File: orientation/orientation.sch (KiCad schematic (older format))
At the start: 8 parts, among them J1 Conn_01x02, J2 Conn_01x04, SW1 SW_SPST, U1 Teensy4.0, U2 STSPIN220, U3 bno055

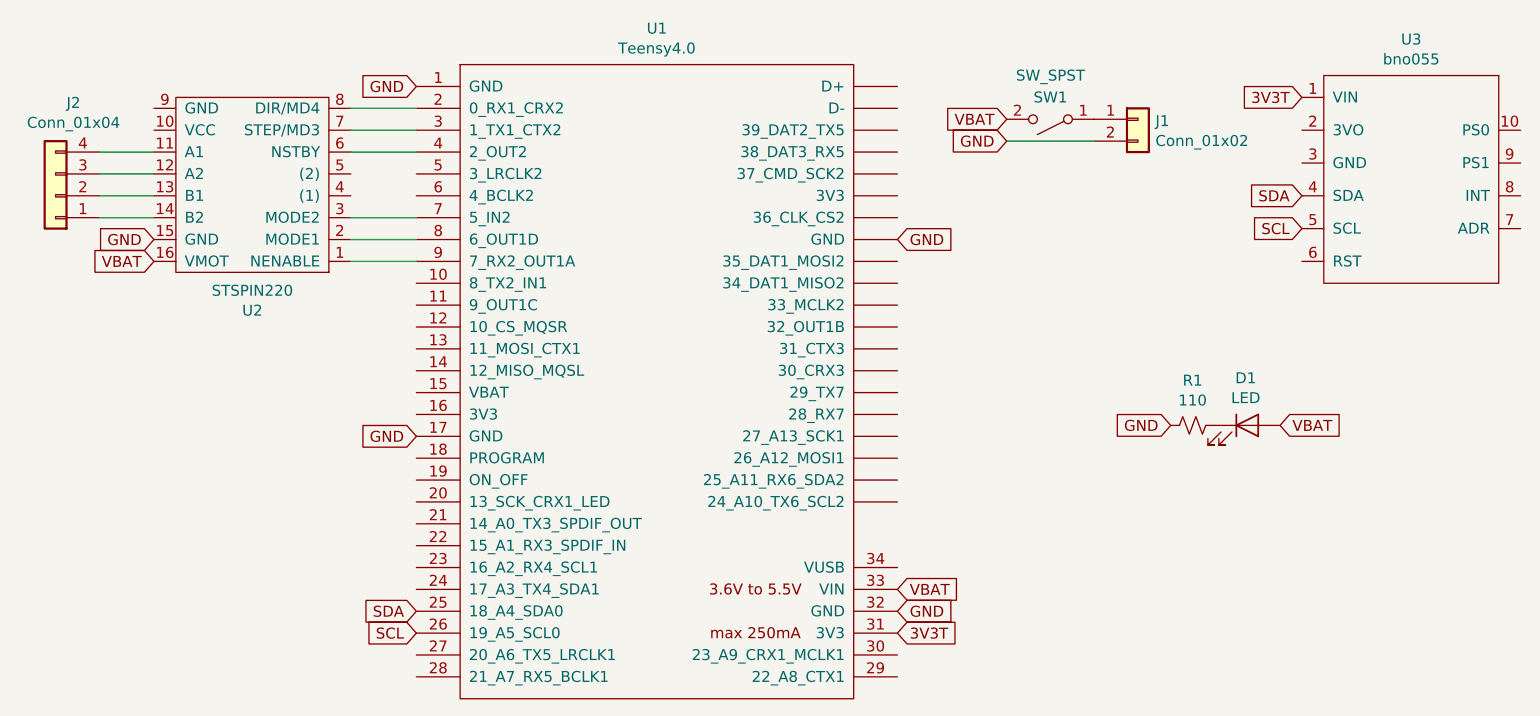
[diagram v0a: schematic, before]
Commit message: misc changes
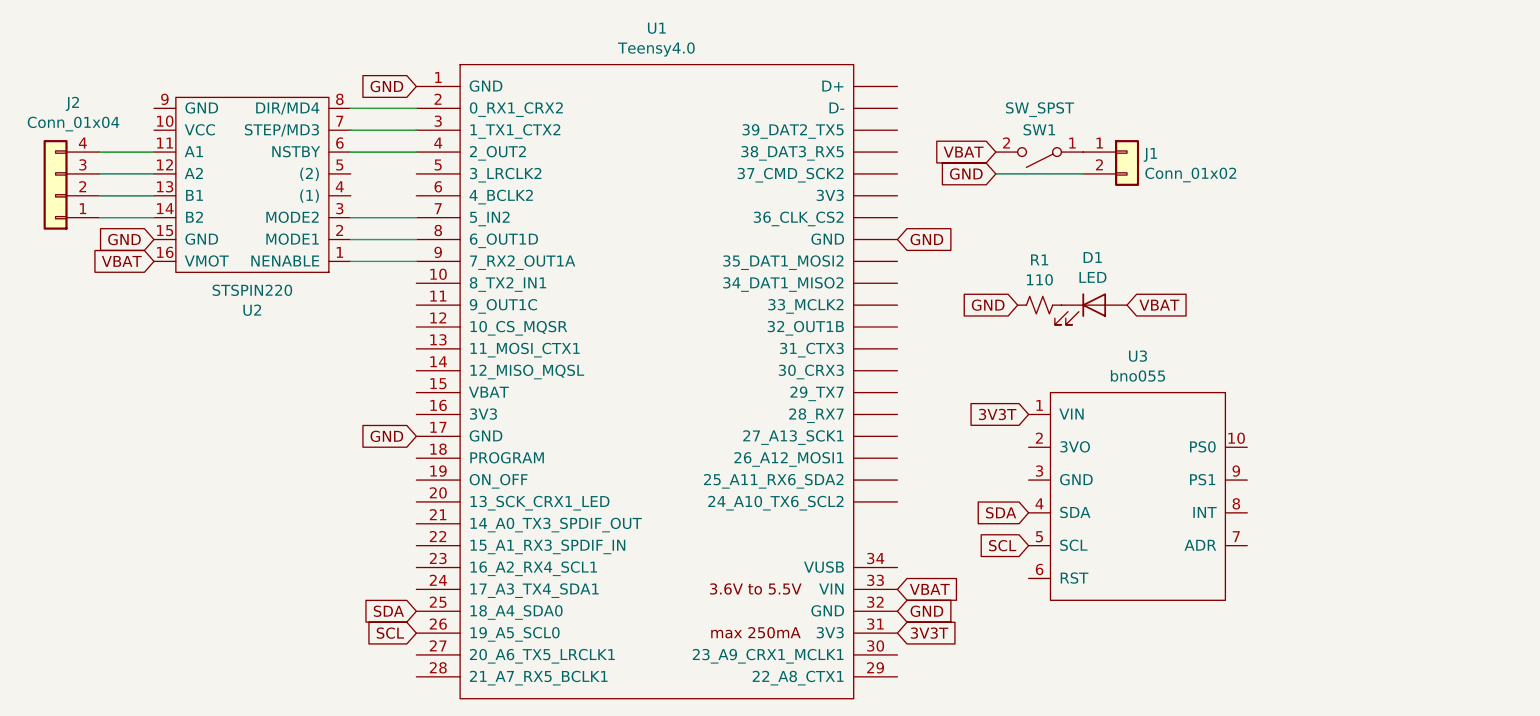
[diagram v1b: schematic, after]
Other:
- moved on the sheet: D1, J1, R1, SW1, U3
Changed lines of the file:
@@
 L NUSTARS:bno055 U3
 U 1 1 5E1EF17C
-P 6550 2300
-F 0 "U3" H 6950 2465 50  0000 C CNN
-F 1 "bno055" H 6950 2374 50  0000 C CNN
-F 2 "NUSTARS:bno055" H 6900 2450 50  0001 C CNN
-F 3 "" H 6900 2450 50  0001 C CNN
-	1    6550 2300
+P 5300 3750
+F 0 "U3" H 5700 3915 50  0000 C CNN
+F 1 "bno055" H 5700 3824 50  0000 C CNN
+F 2 "NUSTARS:bno055" H 5650 3900 50  0001 C CNN
+F 3 "" H 5650 3900 50  0001 C CNN
+	1    5300 3750
 	1    0    0    -1
 $EndComp
@@
 L Connector_Generic:Conn_01x02 J1
 U 1 1 5E1EFEDF
-P 5700 2500
-F 0 "J1" H 5780 2492 50  0000 L CNN
-F 1 "Conn_01x02" H 5780 2401 50  0000 L CNN
-F 2 "Connector_JST:JST_PH_B2B-PH-K_1x02_P2.00mm_Vertical" H 5700 2500 50  0001 C CNN
-F 3 "~" H 5700 2500 50  0001 C CNN
-	1    5700 2500
+P 5650 2650
+F 0 "J1" H 5730 2642 50  0000 L CNN
+F 1 "Conn_01x02" H 5730 2551 50  0000 L CNN
+F 2 "Connector_JST:JST_PH_B2B-PH-K_1x02_P2.00mm_Vertical" H 5650 2650 50  0001 C CNN
+F 3 "~" H 5650 2650 50  0001 C CNN
+	1    5650 2650
 	1    0    0    -1
 $EndComp
@@
 Text GLabel 2400 4750 0    50   Input ~ 0
 SDA
-Text GLabel 5100 2500 0    50   Input ~ 0
+Text GLabel 5050 2650 0    50   Input ~ 0
 VBAT
-Text GLabel 5100 2600 0    50   Input ~ 0
+Text GLabel 5050 2750 0    50   Input ~ 0
 GND
 Text GLabel 4600 4850 2    50   Input ~ 0
 3V3T
-Text GLabel 6450 2400 0    50   Input ~ 0
+Text GLabel 5200 3850 0    50   Input ~ 0
 3V3T
-Text GLabel 6450 2850 0    50   Input ~ 0
+Text GLabel 5200 4300 0    50   Input ~ 0
 SDA
-Text GLabel 6450 3000 0    50   Input ~ 0
+Text GLabel 5200 4450 0    50   Input ~ 0
 SCL
 Text GLabel 2400 2350 0    50   Input ~ 0
@@
 L Switch:SW_SPST SW1
 U 1 1 5E1530D8
-P 5300 2500
-F 0 "SW1" H 5300 2400 50  0000 C CNN
-F 1 "SW_SPST" H 5300 2300 50  0000 C CNN
-F 2 "NUSTARS:GF-123-0054" H 5300 2500 50  0001 C CNN
-F 3 "~" H 5300 2500 50  0001 C CNN
-	1    5300 2500
+P 5250 2650
+F 0 "SW1" H 5250 2550 50  0000 C CNN
+F 1 "SW_SPST" H 5250 2450 50  0000 C CNN
+F 2 "NUSTARS:GF-123-0054" H 5250 2650 50  0001 C CNN
+F 3 "~" H 5250 2650 50  0001 C CNN
+	1    5250 2650
 	-1   0    0    1
 $EndComp
 Wire Wire Line
-	5500 2600 5100 2600
+	5450 2750 5050 2750
 $Comp
 L Device:LED D1
 U 1 1 5E15F99C
-P 6200 3900
-F 0 "D1" H 6193 4116 50  0000 C CNN
-F 1 "LED" H 6193 4025 50  0000 C CNN
-F 2 "LED_SMD:LED_1206_3216Metric_Pad1.42x1.75mm_HandSolder" H 6200 3900 50  0001 C CNN
-F 3 "~" H 6200 3900 50  0001 C CNN
-	1    6200 3900
+P 5500 3350
+F 0 "D1" H 5493 3566 50  0000 C CNN
+F 1 "LED" H 5493 3475 50  0000 C CNN
+F 2 "LED_SMD:LED_1206_3216Metric_Pad1.42x1.75mm_HandSolder" H 5500 3350 50  0001 C CNN
+F 3 "~" H 5500 3350 50  0001 C CNN
+	1    5500 3350
 	1    0    0    -1
 $EndComp
-Text GLabel 6350 3900 2    50   Input ~ 0
+Text GLabel 5650 3350 2    50   Input ~ 0
 VBAT
 $Comp
 L Device:R_Small_US R1
 U 1 1 5E163AC3
-P 5950 3900
-F 0 "R1" V 5745 3900 50  0000 C CNN
-F 1 "110" V 5836 3900 50  0000 C CNN
-F 2 "Resistor_SMD:R_1206_3216Metric_Pad1.42x1.75mm_HandSolder" H 5950 3900 50  0001 C CNN
-F 3 "~" H 5950 3900 50  0001 C CNN
-	1    5950 3900
+P 5250 3350
+F 0 "R1" V 5045 3350 50  0000 C CNN
+F 1 "110" V 5136 3350 50  0000 C CNN
+F 2 "Resistor_SMD:R_1206_3216Metric_Pad1.42x1.75mm_HandSolder" H 5250 3350 50  0001 C CNN
+F 3 "~" H 5250 3350 50  0001 C CNN
+	1    5250 3350
 	0    1    1    0
 $EndComp
-Text GLabel 5850 3900 0    50   Input ~ 0
+Text GLabel 5150 3350 0    50   Input ~ 0
 GND
 $EndSCHEMATC
